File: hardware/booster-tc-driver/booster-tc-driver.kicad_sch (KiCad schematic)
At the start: 61 parts, among them J1 62201021121, J2 EHT-105-01-S-D, J3 22-23-2021, Q1 T2N7002AK, Q2 SI4056ADY-T1-GE3, Q3 SI4056ADY-T1-GE3, U1 STM32F405RGTx, U2 LT1963AxST-3.3, U3 MAX9202ESD+, U4 IF-D95T << must be T, U6 IF-D95T << must be T, U7 TC7662Bx0A

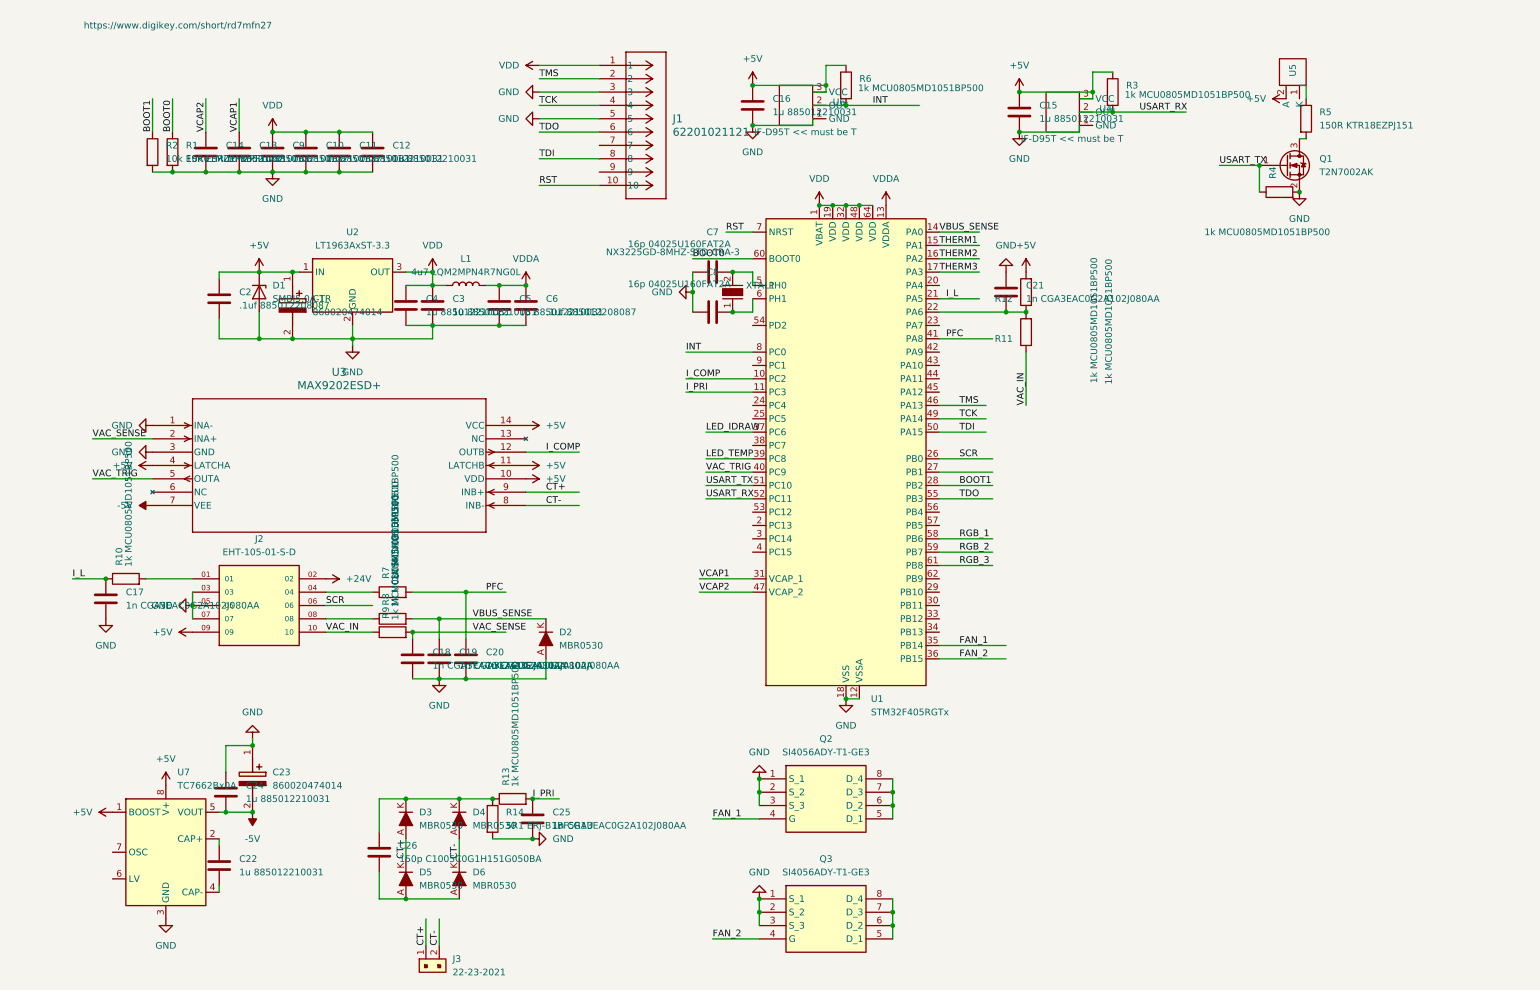
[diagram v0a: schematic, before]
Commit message: driver pcb
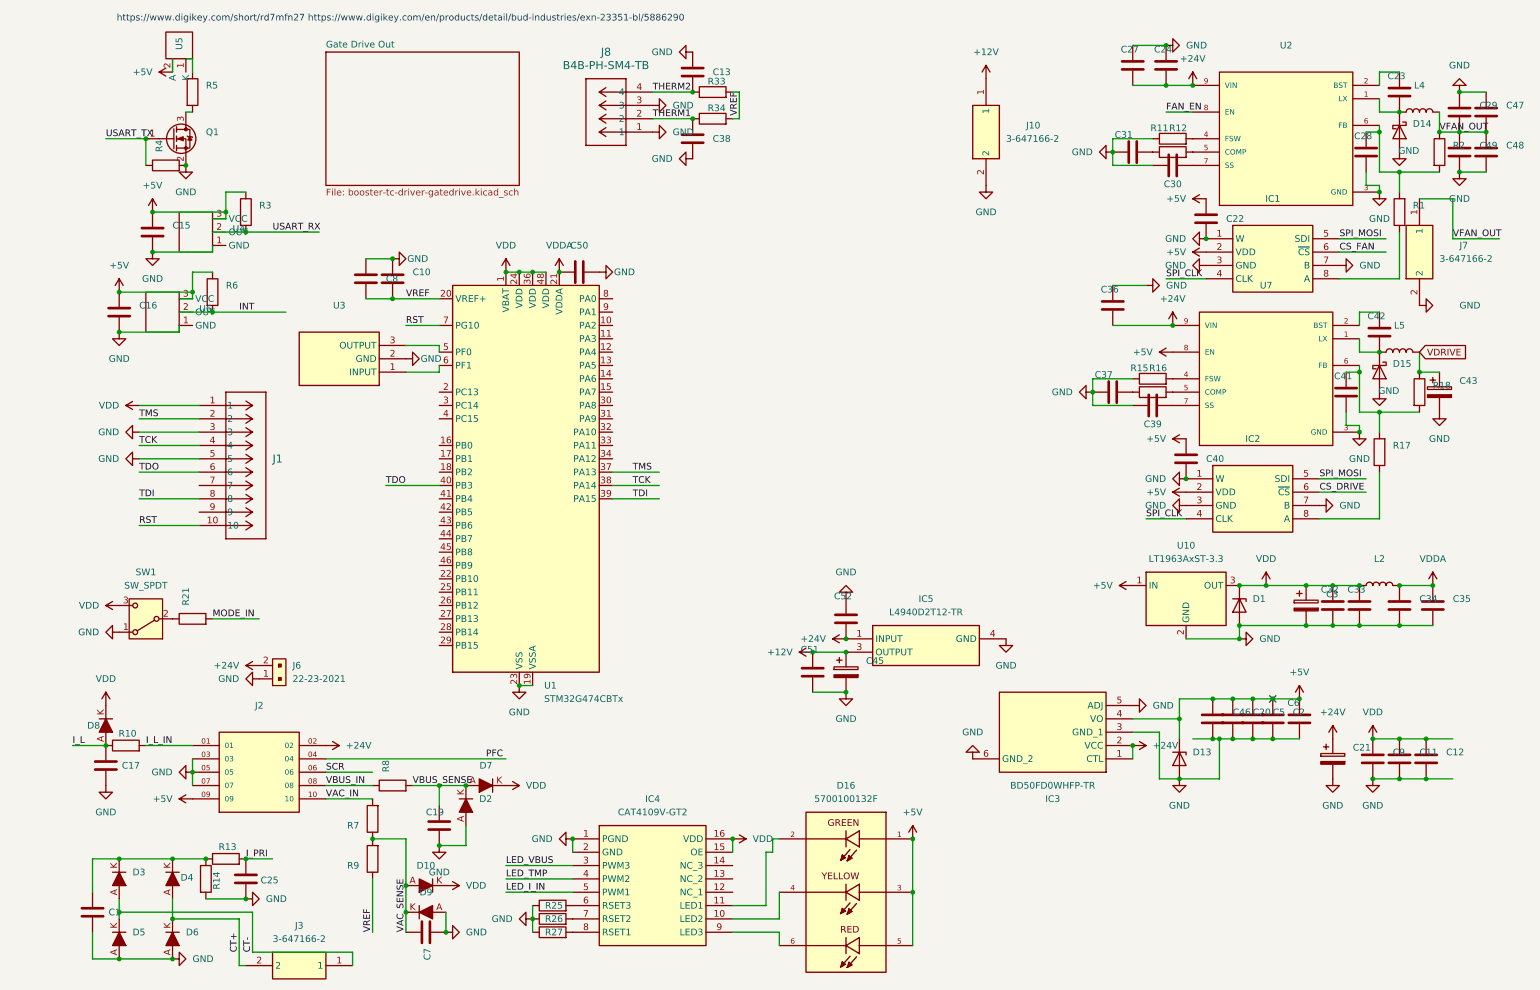
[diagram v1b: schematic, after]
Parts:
- removed C1, C23: 860020474014, Library:CAPPRD350W52D800H1300, symbol New_Library:860020474014
- removed C14, C3, C4: 1u 885012210031, Capacitor_SMD:C_1812_4532Metric_Pad1.57x3.40mm_HandSolder, symbol Device:C
- removed C18, C21: 1n CGA3EAC0G2A102J080AA, Capacitor_SMD:C_0603_1608Metric_Pad1.08x0.95mm_HandSolder, symbol Device:C
- removed C26: 150p C1005C0G1H151G050BA, Capacitor_SMD:C_01005_0402Metric_Pad0.57x0.30mm_HandSolder, symbol Device:C
- removed J3: 22-23-2021, digikey-footprints:PinHeader_1x2_P2.54mm_Drill1.02mm, symbol dk_Rectangular-Connectors-Headers-Male-Pins:22-23-2021
- removed L1: 4u7 LQM2MPN4R7NG0L, Inductor_SMD:L_Murata_DFE201610P, symbol Device:L
- removed Q2, Q3: SI4056ADY-T1-GE3, Library:SOIC127P600X175-8N, symbol SI4056ADY-T1-GE3:SI4056ADY-T1-GE3
- removed U1: STM32F405RGTx, Package_QFP:LQFP-64_10x10mm_P0.5mm, symbol MCU_ST_STM32F4:STM32F405RGTx
- removed U2: LT1963AxST-3.3, Package_TO_SOT_SMD:SOT-223-3_TabPin2, symbol Regulator_Linear:LT1963AxST-3.3
- removed U3: MAX9202ESD+, Library:21-0041B_14-L, symbol 2024-07-01_19-30-11:MAX9202ESD+
- removed U7: TC7662Bx0A, Package_SO:SOIC-8_3.9x4.9mm_P1.27mm, symbol Converter_DCDC:TC7662Bx0A
- removed XTAL1: NX3225GD-8MHZ-STD-CRA-3, digikey-footprints:SMD-2_3.2x2.5mm, symbol dk_Crystals:NX3225GD-8MHZ-STD-CRA-3
- added C1, C31, C37: 1n CGA3EAC0G2A102J080AA, Capacitor_SMD:C_0603_1608Metric_Pad1.08x0.95mm_HandSolder, symbol Device:C
- added C21, C3, C43, C45: 330u 860020575013, Library:860020575013, symbol Device:C_Polarized
- added C23, C27, C28, C32, C33, C35, C36, C40, C41, C42, C51, C52: .1uf 885012208087, Capacitor_SMD:C_1206_3216Metric_Pad1.33x1.80mm_HandSolder, symbol Device:C
- added C29, C34, C46, C47, C48, C49: 2u2 C3225X7R1H225K250AB, Capacitor_SMD:C_1210_3225Metric_Pad1.33x2.70mm_HandSolder, symbol Device:C
- added C30, C39: 22n VJ0805Y223KBBBE31, Capacitor_SMD:C_0805_2012Metric_Pad1.18x1.45mm_HandSolder, symbol Device:C
- added C38, C50: .1uf C0603C104K3RECTU, Capacitor_SMD:C_0603_1608Metric_Pad1.08x0.95mm_HandSolder, symbol Device:C
- added D10, D7, D8, D9: MBR0530, digikey-footprints:SOD-123, symbol dk_Diodes-Rectifiers-Single:1N5819HW-7-F
- added D13: SMBJ5.0A-TR, kicad-libraries-master:DO-214AA, symbol Device:D_Zener
- added D14, D15: PMEG4050EP, Diode_SMD:D_SOD-128, symbol Diode:PMEG4050EP
- added D16: 5700100132F, Library:LED_5700100132F, symbol 5700100132F:5700100132F
- added IC1, IC2: AD5160BRJZ5-RL7, Library:SOT65P280X145-8N, symbol New_Library:AD5160BRJZ5-RL7
- added IC3: BD50FD0WHFP-TR, Library:BD50FD0WHFPTR, symbol New_Library:BD50FD0WHFP-TR
- added IC4: CAT4109V-GT2, Library:CAT4109V-GT2, symbol New_Library:CAT4109V-GT2
- added IC5: L4940D2T12-TR, Library:L4940D2T12-TR, symbol New_Library:L4940D2T12-TR
- added J10, J3, J7: 3-647166-2, Library:36471662, symbol New_Library:3-647166-2
- added J6: 22-23-2021, digikey-footprints:PinHeader_1x2_P2.54mm_Drill1.02mm, symbol dk_Rectangular-Connectors-Headers-Male-Pins:22-23-2021
- added J8: B4B-PH-SM4-TB, Library:CONN_B4B-PH-SM4-TB_JST, symbol New_Library:B4B-PH-SM4-TB
- added L2: 4u7 LQM2MPN4R7NG0L, Inductor_SMD:L_Murata_DFE201610P, symbol Device:L
- added L4, L5: 22u 7443551221, Library:7443551221, symbol Device:L
- added R15: 47k CRCW080547K0FKEA, Resistor_SMD:R_0805_2012Metric_Pad1.20x1.40mm_HandSolder, symbol Device:R
- added R16: 470k CRCW0805470KFKTA, Resistor_SMD:R_0805_2012Metric_Pad1.20x1.40mm_HandSolder, symbol Device:R
- added R17: 3k CRCW08053K00FKTA, Resistor_SMD:R_0805_2012Metric_Pad1.20x1.40mm_HandSolder, symbol Device:R
- added R18: 82k CRCW080582K0FKEA, Resistor_SMD:R_0805_2012Metric_Pad1.20x1.40mm_HandSolder, symbol Device:R
- added R21: 1k MCU0805MD1051BP500, Resistor_SMD:R_0805_2012Metric_Pad1.20x1.40mm_HandSolder, symbol Device:R
- added R25, R26, R27: 24k9 CRCW060324K9FKEA, Resistor_SMD:R_0603_1608Metric_Pad0.98x0.95mm_HandSolder, symbol Device:R
- added R33, R34: 10k CRCW080510K0DHEAP, Resistor_SMD:R_0805_2012Metric_Pad1.20x1.40mm_HandSolder, symbol Device:R
- added SW1: SW_SPDT, Library:B12JV, symbol Switch:SW_SPDT
- added U1: STM32G474CBTx, Package_QFP:LQFP-48_7x7mm_P0.5mm, symbol MCU_ST_STM32G4:STM32G474CBTx
- added U10: LT1963AxST-3.3, Package_TO_SOT_SMD:SOT-223-3_TabPin2, symbol Regulator_Linear:LT1963AxST-3.3
- added U2, U7: AOZ1284PI, Package_SO:SOIC-8-1EP_3.9x4.9mm_P1.27mm_EP2.29x3mm, symbol New_Library:AOZ1284PI
- added U3: CSTNE8M00G550000R0, Library:CSTNE16M0V530000R0, symbol New_Library:CSTNE8M00G550000R0
- C10, C11, C12, C13, C9: value 1u 885012210031 -> .1uf C0603C104K3RECTU; footprint Capacitor_SMD:C_1812_4532Metric_Pad1.57x3.40mm_HandSolder -> Capacitor_SMD:C_0603_1608Metric_Pad1.08x0.95mm_HandSolder
- C15, C16, C5: value 1u 885012210031 -> 2u2 C3225X7R1H225K250AB; footprint Capacitor_SMD:C_1812_4532Metric_Pad1.57x3.40mm_HandSolder -> Capacitor_SMD:C_1210_3225Metric_Pad1.33x2.70mm_HandSolder
- C2: value .1uf 885012208087 -> 2u2 C3225X7R1H225K250AB; footprint Capacitor_SMD:C_1206_3216Metric_Pad1.33x1.80mm_HandSolder -> Capacitor_SMD:C_1210_3225Metric_Pad1.33x2.70mm_HandSolder
- C20: value 1n CGA3EAC0G2A102J080AA -> 2u2 C3225X7R1H225K250AB; footprint Capacitor_SMD:C_0603_1608Metric_Pad1.08x0.95mm_HandSolder -> Capacitor_SMD:C_1210_3225Metric_Pad1.33x2.70mm_HandSolder
- C22, C24: value 1u 885012210031 -> .1uf 885012208087; footprint Capacitor_SMD:C_1812_4532Metric_Pad1.57x3.40mm_HandSolder -> Capacitor_SMD:C_1206_3216Metric_Pad1.33x1.80mm_HandSolder
- C7: value 16p 04025U160FAT2A -> 1n CGA3EAC0G2A102J080AA; footprint Capacitor_SMD:C_0402_1005Metric_Pad0.74x0.62mm_HandSolder -> Capacitor_SMD:C_0603_1608Metric_Pad1.08x0.95mm_HandSolder
- C8: value 16p 04025U160FAT2A -> 1u C1206C105K5RACTU; footprint Capacitor_SMD:C_0402_1005Metric_Pad0.74x0.62mm_HandSolder -> Capacitor_SMD:C_1206_3216Metric_Pad1.33x1.80mm_HandSolder
- D1: value SMBJ5.0A-TR -> SMBJ3V3
- D2: MPN 1N5819HW-7-F -> MBR0530
- D3, D4, D5, D6: value MBR0530 -> 1N5819HW-7-F
- R1: value 10k ESR01MZPF1002 -> 3k CRCW08053K00FKTA; footprint Resistor_SMD:R_0402_1005Metric_Pad0.72x0.64mm_HandSolder -> Resistor_SMD:R_0805_2012Metric_Pad1.20x1.40mm_HandSolder
- R11: value 1k MCU0805MD1051BP500 -> 47k CRCW080547K0FKEA
- R12: value 1k MCU0805MD1051BP500 -> 470k CRCW0805470KFKTA
- R2: value 10k ESR01MZPF1002 -> 82k CRCW080582K0FKEA; footprint Resistor_SMD:R_0402_1005Metric_Pad0.72x0.64mm_HandSolder -> Resistor_SMD:R_0805_2012Metric_Pad1.20x1.40mm_HandSolder
- U5: value ~ -> IF-E96E
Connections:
- net -5V is gone; now on net +24V: C24.2
- net VCAP1 is gone; now on net THERM2: C13.1
- net +24V: now also C21.1, C27.2, C36.2, C52.2, IC3.1 (CTL), IC3.2 (VCC), IC5.1 (INPUT), J6.2, U2.9 (VIN), U7.9 (VIN)
- net +5V: now also C20.1, C22.2, C5.1, C6.1, U5.2 (A), C40.2, C46.1, D13.1 (K), D16.1, D16.3, D16.5, IC1.2 (VDD), IC2.2 (VDD), IC3.4 (VO), U10.1 (IN), U7.8 (EN); no longer D1.1 (K), R12.2
- net CT+: now also D4.A, D6.K, J3.2; no longer D3.A, D5.K
- net CT-: now also D3.A, D5.K, J3.1; no longer D4.A, D6.K
- net GND: now also C10.1, C22.1, C7.2, D5.A, D6.A, R11.1, C1.2, C21.2, C27.1, C28.2, C29.1, C3.2, C30.2, C31.1, C32.2, C33.2, C34.2, C35.2, C36.1, C37.1, C38.1, C39.2, C40.1, C41.2, C43.2, C45.2, C46.2, C47.1, C48.2, C49.2, C50.2, C51.2, C52.1, D13.2 (A), D14.2 (A), D15.2 (A), D9.A, IC1.1 (W), IC1.3 (GND), IC1.7 (B), IC2.1 (W), IC2.3 (GND), IC2.7 (B), IC3.3 (GND_1), IC3.5 (ADJ), IC3.6 (GND_2), IC4.1 (PGND), IC4.2 (GND), IC5.4 (GND), J10.2, J6.1, J7.2, J8.1, J8.3, R15.1, R25.1, R26.1, R27.1, SW1.1 (A), U1.19 (VSSA), U1.23 (VSS), U1.35 (VSS), U1.47 (VSS), U10.2 (GND), U2.3 (GND), U3.2 (GND), U7.3 (GND); no longer C10.2, C7.1, R1.2, R2.2
- net I_L: now also D8.A
- net PFC: now also J2.04; no longer C20.1, R7.2
- net RST: now also U1.7 (PG10)
- net TCK: now also U1.38 (PA14)
- net TDI: now also U1.39 (PA15)
- net TDO: now also U1.40 (PB3)
- net THERM1: now also C38.2, J8.2, R34.1
- net THERM2: now also J8.4, R33.1
- net TMS: now also U1.37 (PA13)
- net VAC_IN: now also R7.2; no longer R11.1, R9.1
- net VAC_SENSE: now also C7.1, R7.1, D10.A, D9.K
- net VBUS_SENSE: now also D7.A
- net VDD: now also D1.1 (K), C3.1, C32.1, C33.1, D10.K, D7.K, D8.K, IC4.15 (OE), IC4.16 (VDD), L2.1, SW1.3 (C), U1.1 (VBAT), U1.24 (VDD), U1.36 (VDD), U1.48 (VDD), U10.3 (OUT); no longer C10.1
- net VDDA: now also C34.1, C35.1, C50.1, L2.2, U1.21 (VDDA); no longer C5.1, C6.1
- net VBUS_IN: now reaches J2.08, R8.1
- net at D3.K, D4.K, R13.1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: now also C1.1
- net at R12.1: now also C31.2; no longer R11.2
- net VREF: now reaches C8.2
- net VREF: now also C10.2, R9.1, R33.2, R34.2, U1.20 (VREF+)
- net I_L_IN: now reaches J2.01, R10.2
- net BOOT0: no longer names the net of R1.1
- net BOOT0: now also IC1.8 (A)
- net BOOT1 renamed VFAN_OUT
- net VFAN_OUT: now also C29.2, C47.2, C48.1, C49.1, J7.1, L4.2
- new net: IC2.8 (A), R17.1
- new net: C41.1, R17.2, R18.2, U7.6 (FB)
- new net: R21.1, SW1.2 (B)
- new net: R12.2, U2.5 (COMP)
- new net: U1.5 (PF0), U3.3 (OUTPUT)
- new net: U1.6 (PF1), U3.1 (INPUT)
- new net: R15.2, U7.4 (FSW)
- new net: D16.4, IC4.10 (LED2)
- new net: D16.2, IC4.11 (LED1)
- new net: IC4.6 (RSET3), R25.2
- new net: IC4.7 (RSET2), R26.2
- new net: IC4.8 (RSET1), R27.2
- new net: D16.6, IC4.9 (LED3)
- new net: C42.1, U7.2 (BST)
- new net: C42.2, D15.1 (K), L5.1, U7.1 (LX)
- new net: C37.2, R16.1
- new net: R16.2, U7.5 (COMP)
- new net: C28.1, R1.2, R2.2, U2.6 (FB)
- new net: C23.1, U2.2 (BST)
- new net: C23.2, D14.1 (K), L4.1, U2.1 (LX)
- new net: C39.1, U7.7 (SS)
- new net: C30.1, U2.7 (SS)
- new net: R11.2, U2.4 (FSW)
- new net +12V: C45.1, C51.1, IC5.3 (OUTPUT), J10.1
- new net CS_DRIVE: IC2.6 (~{CS})
- new net CS_FAN: IC1.6 (~{CS})
- new net FAN_EN: U2.8 (EN)
- new net LED_I_IN: IC4.5 (PWM1)
- new net LED_TMP: IC4.4 (PWM2)
- new net LED_VBUS: IC4.3 (PWM3)
- new net MODE_IN: R21.2
- new net SPI_CLK: IC1.4 (CLK), IC2.4 (CLK)
- new net SPI_MOSI: IC1.5 (SDI), IC2.5 (SDI)
- new net VDRIVE: C43.1, L5.2, R18.1
- no-connect marks 0 -> 1
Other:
- added sheet Gate Drive Out (booster-tc-driver-gatedrive.kicad_sch)
- note added: "https://www.digikey.com/short/rd7mfn27 https://www.digikey.com/en/products/detail/bud-industries/exn-23351-bl/5886290"
- note removed: "https://www.digikey.com/short/rd7mfn27"
- moved on the sheet: C17, C19, C25, D2, D3, D4, D5, D6, J1, J2, Q1, R10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
